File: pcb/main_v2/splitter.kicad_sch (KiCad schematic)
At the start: 15 parts, among them IC601 PSA4-5043+, IC602 PSA4-5043+, U601 PD0922J5050D2HF, U602 XMB0220K1-50100G

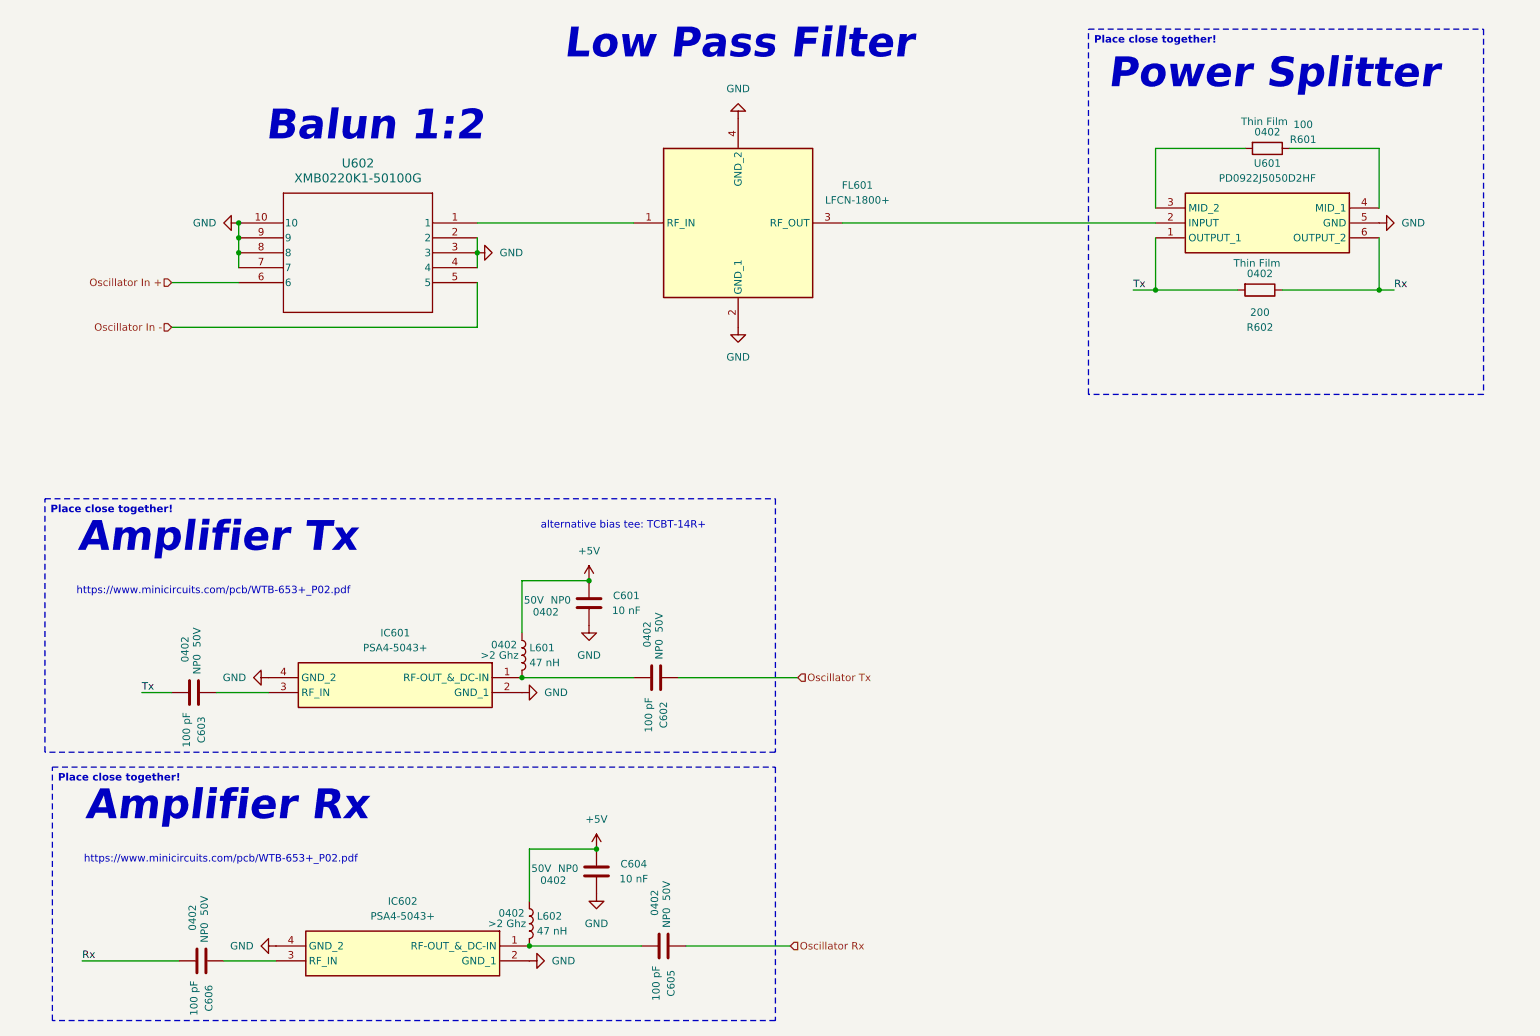
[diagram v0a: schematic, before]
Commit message: finished layout
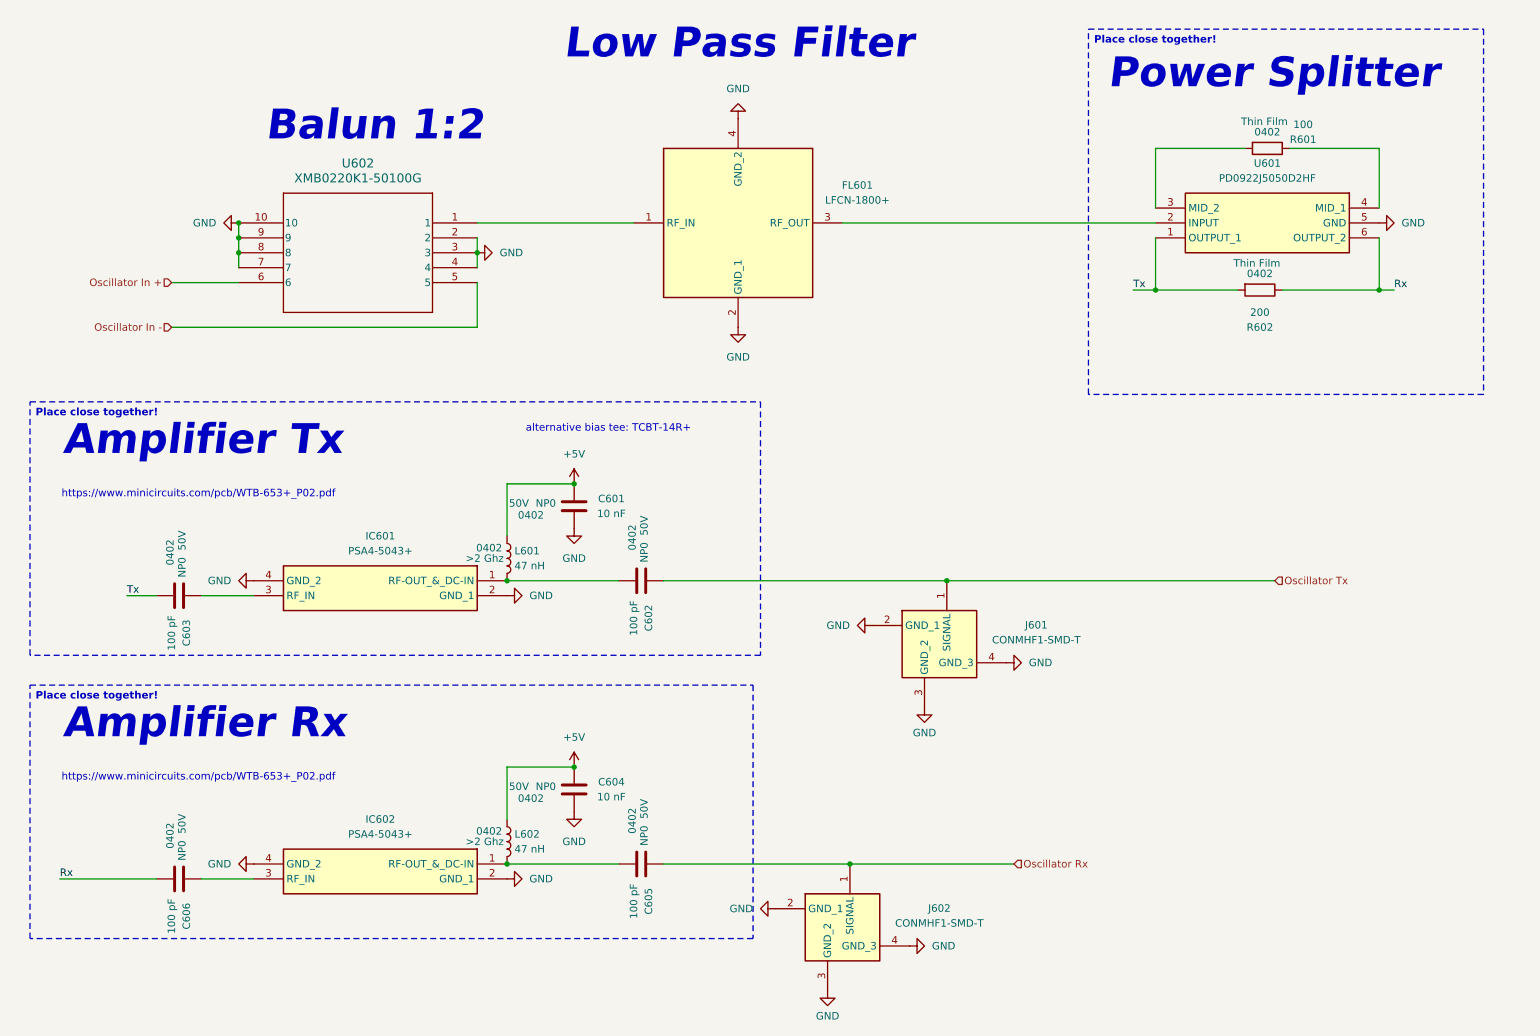
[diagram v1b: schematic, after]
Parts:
- added J601, J602: CONMHF1-SMD-T, My Footprints:CONMHF1SMDT, symbol My Symbols:CONMHF1-SMD-T
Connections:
- net GND: now also J601.2 (GND_1), J601.3 (GND_2), J601.4 (GND_3), J602.2 (GND_1), J602.3 (GND_2), J602.4 (GND_3)
- net Oscillator Rx: now also J602.1 (SIGNAL)
- net Oscillator Tx: now also J601.1 (SIGNAL)
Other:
- moved on the sheet: C601, C602, C603, C604, C605, C606, IC601, IC602, L601, L602
